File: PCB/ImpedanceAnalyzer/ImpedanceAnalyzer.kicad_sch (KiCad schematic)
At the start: 0 parts

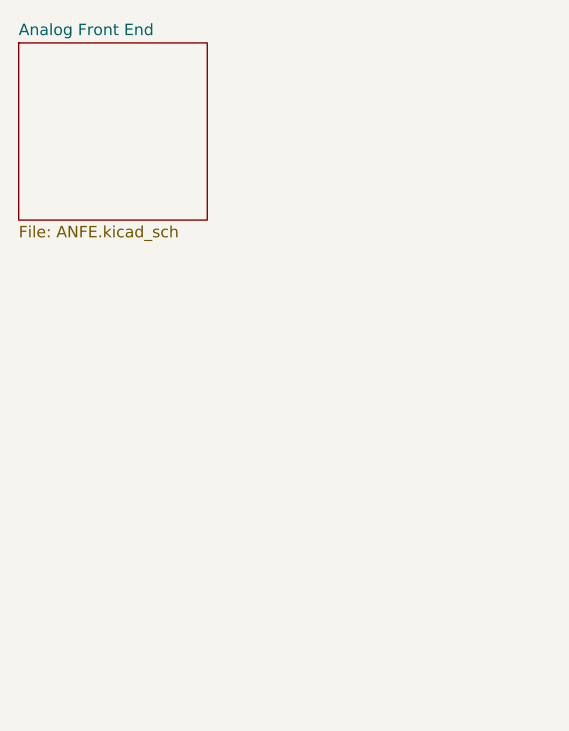
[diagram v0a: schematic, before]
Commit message: test
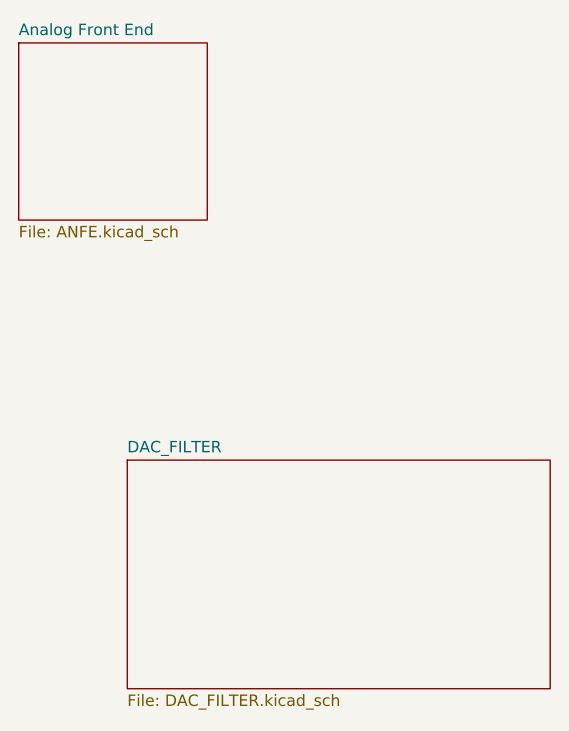
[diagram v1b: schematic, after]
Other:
- added sheet DAC_FILTER (DAC_FILTER.kicad_sch)
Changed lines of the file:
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@@
 	(paper "A4")
+	(sheet
+		(at 88.9 90.17)
+		(size 46.99 25.4)
+		(fields_autoplaced yes)
+		(stroke
+			(width 0.1524)
+			(type solid)
+		)
+		(fill
+			(color 0 0 0 0.0000)
+		)
+		(property "Sheetname" "DAC_FILTER"
+			(at 88.9 89.4584 0)
+			(effects
+				(font
+					(size 1.27 1.27)
+				)
+				(justify left bottom)
+			)
+		)
+		(property "Sheetfile" "DAC_FILTER.kicad_sch"
+			(at 88.9 116.1546 0)
+			(effects
+				(font
+					(size 1.27 1.27)
+				)
+				(justify left top)
+			)
+		)
+		(instances
+			(project "ImpedanceAnalyzer"
+				(path "/08568624-f051-402a-adf3-1b03c2a769ee"
+					(page "3")
+				)
+			)
+		)
+	)
 	(sheet
 		(at 76.835 43.815)

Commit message: filter work
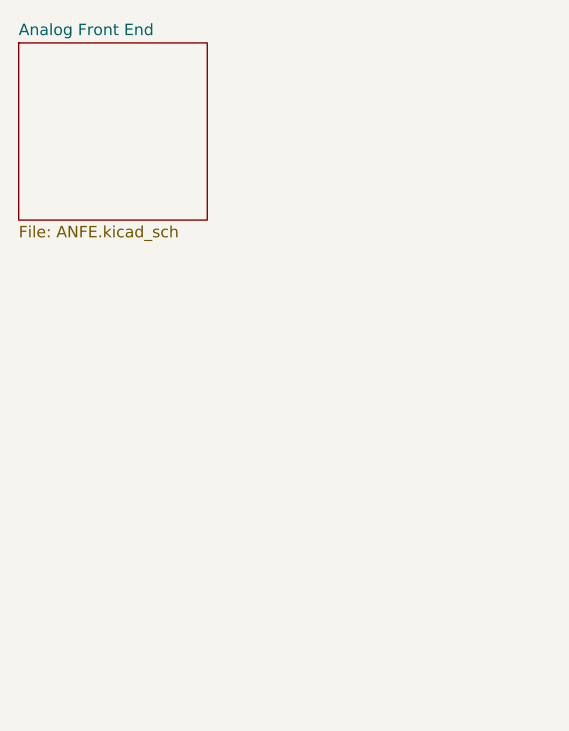
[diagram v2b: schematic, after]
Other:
- removed sheet DAC_FILTER
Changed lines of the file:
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@@
 	(paper "A4")
-	(sheet
-		(at 88.9 90.17)
-		(size 46.99 25.4)
-		(fields_autoplaced yes)
-		(stroke
-			(width 0.1524)
-			(type solid)
-		)
-		(fill
-			(color 0 0 0 0.0000)
-		)
-		(property "Sheetname" "DAC_FILTER"
-			(at 88.9 89.4584 0)
-			(effects
-				(font
-					(size 1.27 1.27)
-				)
-				(justify left bottom)
-			)
-		)
-		(property "Sheetfile" "DAC_FILTER.kicad_sch"
-			(at 88.9 116.1546 0)
-			(effects
-				(font
-					(size 1.27 1.27)
-				)
-				(justify left top)
-			)
-		)
-		(instances
-			(project "ImpedanceAnalyzer"
-				(path "/08568624-f051-402a-adf3-1b03c2a769ee"
-					(page "3")
-				)
-			)
-		)
-	)
 	(sheet
 		(at 76.835 43.815)
